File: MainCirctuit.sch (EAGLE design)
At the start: 9 parts, among them IC1 LM4558N, IC2 NE5532N, IC3 NE5532N, IC4 NE5532N, J4 STEREOSW, J5 STEREOSW

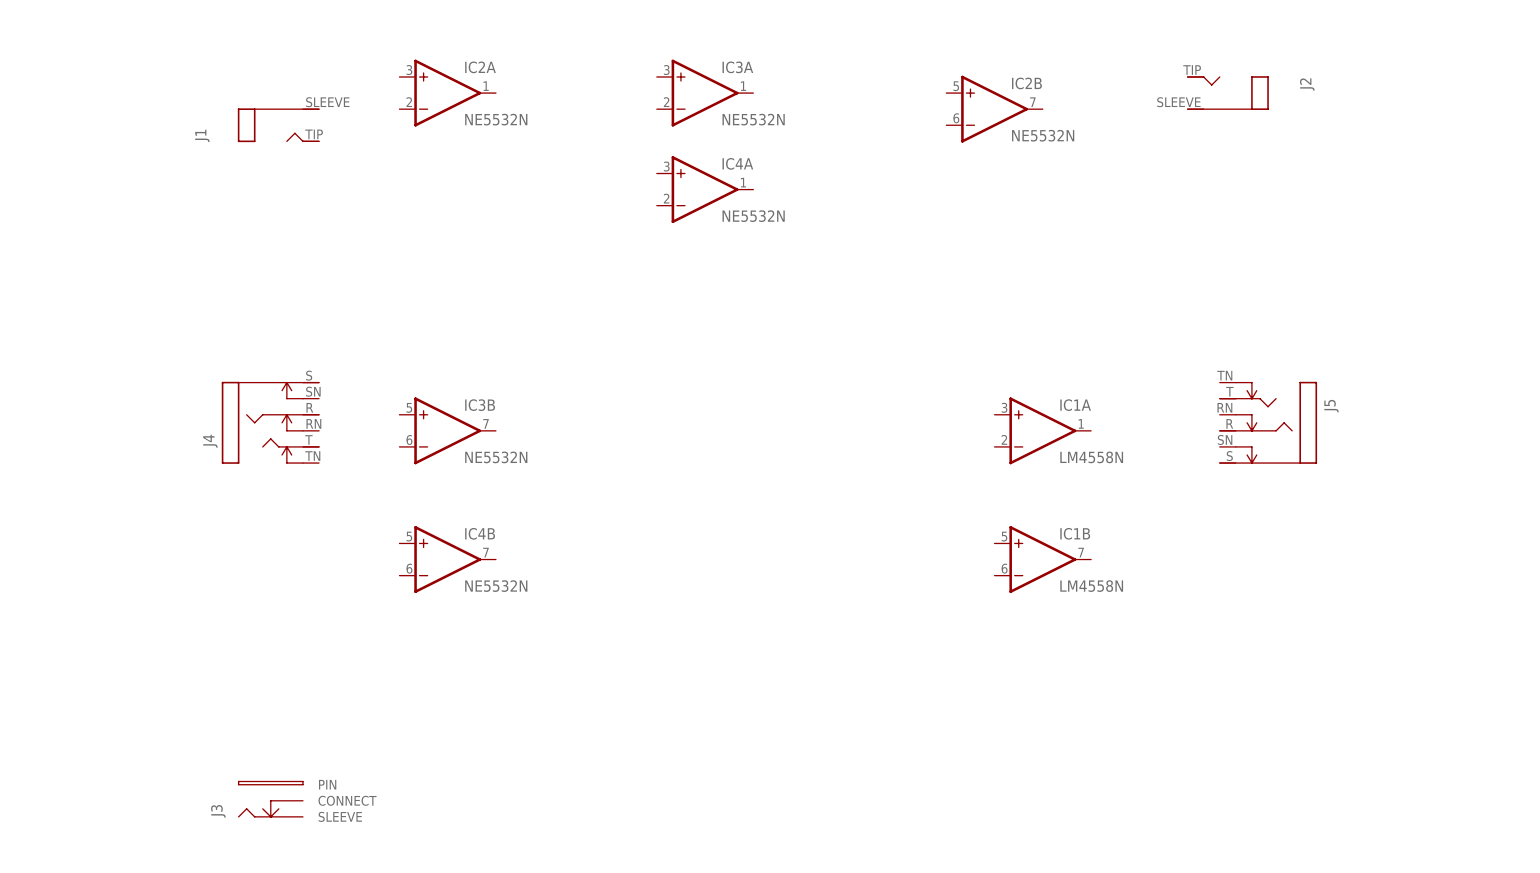
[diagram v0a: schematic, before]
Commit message: Completing circuit
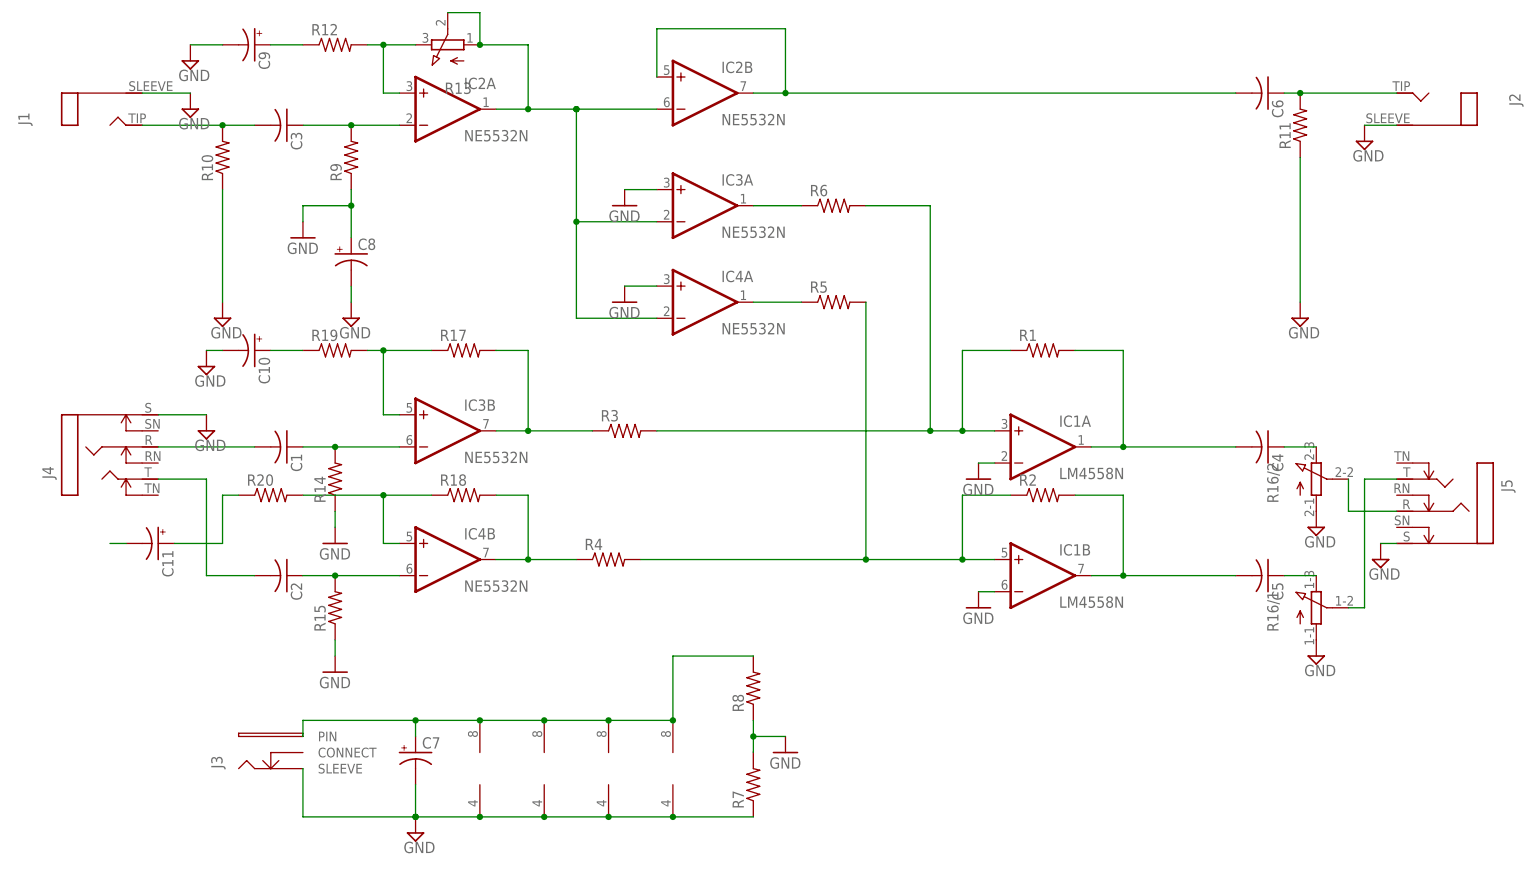
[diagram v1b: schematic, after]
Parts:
- added C1, C2, C3, C4, C5, C6: (no value), resistor:C-US050-025X075
- added C10, C11, C7, C8, C9: (no value), resistor:CPOL-USE2,5-6E
- added R1, R10, R11, R12, R14, R15, R17, R18, R19, R2, R20, R3, R4, R5, R6, R7, R8, R9: (no value), resistor:R-US_0204/7
- added R13: (no value), pot:3RP/1610N
- added R16: (no value), pot:3RP/1610G
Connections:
- new net GND: C10.-, C7.-, C8.+, C8.-, C9.-, IC1A.-IN, IC1B.-IN, IC1P.V-, IC2P.V-, IC3A.+IN, IC3P.V-, IC4A.+IN, IC4P.V-, J1.SLEEVE, J2.SLEEVE, J3.SLEEVE, J4.S, J5.S, R10.1, R11.1, R14.1, R15.1, R16/1.A, R16/2.A, R7.1, R7.2, R8.1, R9.1
- new net N$1: IC3B.OUT, R17.2, R3.1
- new net N$10: C1.1, IC3B.-IN, R14.2
- new net N$11: IC3A.OUT, R6.1
- new net N$12: C2.1, IC4B.-IN, R15.2
- new net N$13: C5.2, IC1B.OUT, R2.2
- new net N$14: J5.R, R16/2.S
- new net N$15: IC2A.OUT, IC2B.-IN, IC3A.-IN, IC4A.-IN, R13.A, R13.S
- new net N$16: C6.2, IC2B.+IN, IC2B.OUT
- new net N$17: C3.2, J1.TIP, R10.2
- new net N$18: C3.1, IC2A.-IN, R9.2
- new net N$19: C6.1, J2.TIP, R11.2
- new net N$2: IC4B.OUT, R18.2, R4.1
- new net N$20: C7.+, IC1P.V+, IC2P.V+, IC3P.V+, IC4P.V+, J3.PIN, R8.2
- new net N$21: C9.+, R12.1
- new net N$22: IC2A.+IN, R12.2, R13.E
- new net N$23: C4.1, R16/2.E
- new net N$24: C5.1, R16/1.E
- new net N$25: IC4B.+IN, R18.1, R20.2
- new net N$26: IC3B.+IN, R17.1, R19.2
- new net N$27: C10.+, R19.1
- new net N$28: C11.+, R20.1
- new net N$29: C11.-
- new net N$3: IC4A.OUT, R5.1
- new net N$4: J5.T, R16/1.S
- new net N$5: IC1B.+IN, R2.1, R4.2, R5.2
- new net N$6: IC1A.+IN, R1.1, R3.2, R6.2
- new net N$7: C4.2, IC1A.OUT, R1.2
- new net N$8: C2.2, J4.T
- new net N$9: C1.2, J4.R
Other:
- moved on the sheet: IC1A, IC1B, IC2A, IC2B, IC3A, IC4A, J1, J2, J3, J4, J5
